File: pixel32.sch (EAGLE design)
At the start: 66 parts, among them CON1 DS1066-07M-SIDE, CON2 DS1066-07M-SIDE, CON3 PINHEAD_1X02-2.54, CON4 PINHEAD_1X01-2.54, CON5 PINHEAD_1X01-2.54, CON6 PINHEAD_1X01-2.54, CON7 PINHEAD_1X01-2.54, IC1 STM32F030K6TX-LQFP32(7X7), IC3 ST3485SOIC8, IC6 MC74VHC1GT125, IC7 MC74VHC1GT125, IC8 LM317

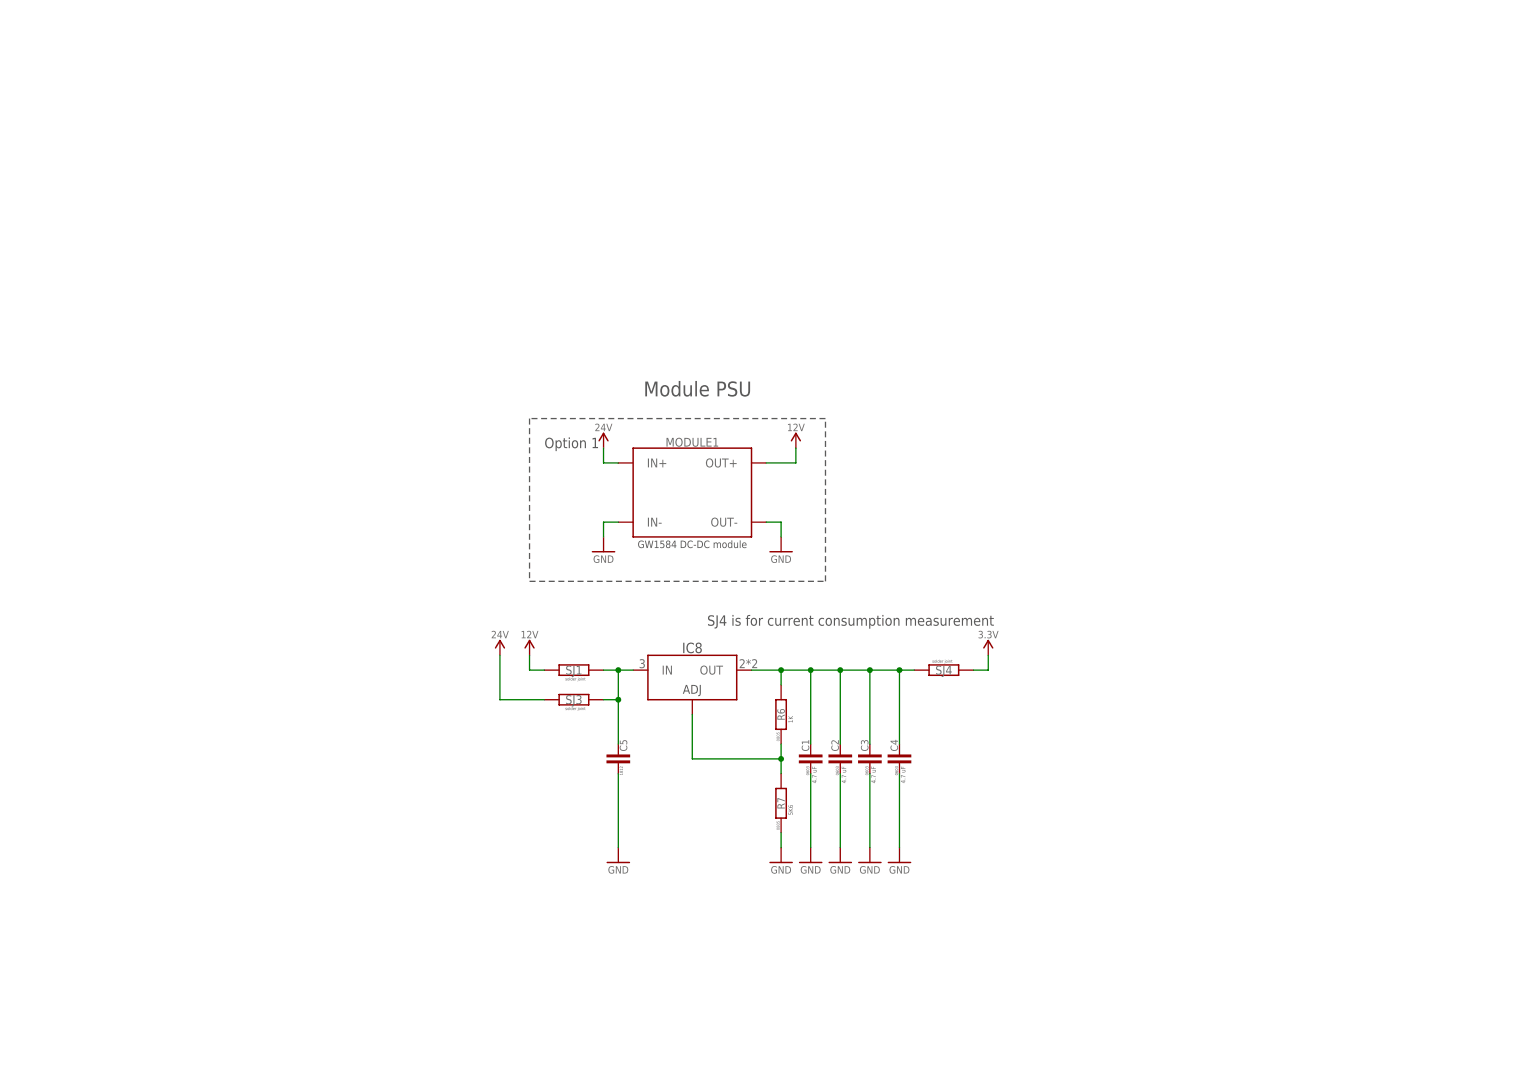
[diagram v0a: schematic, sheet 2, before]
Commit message: PCB Finalization #2
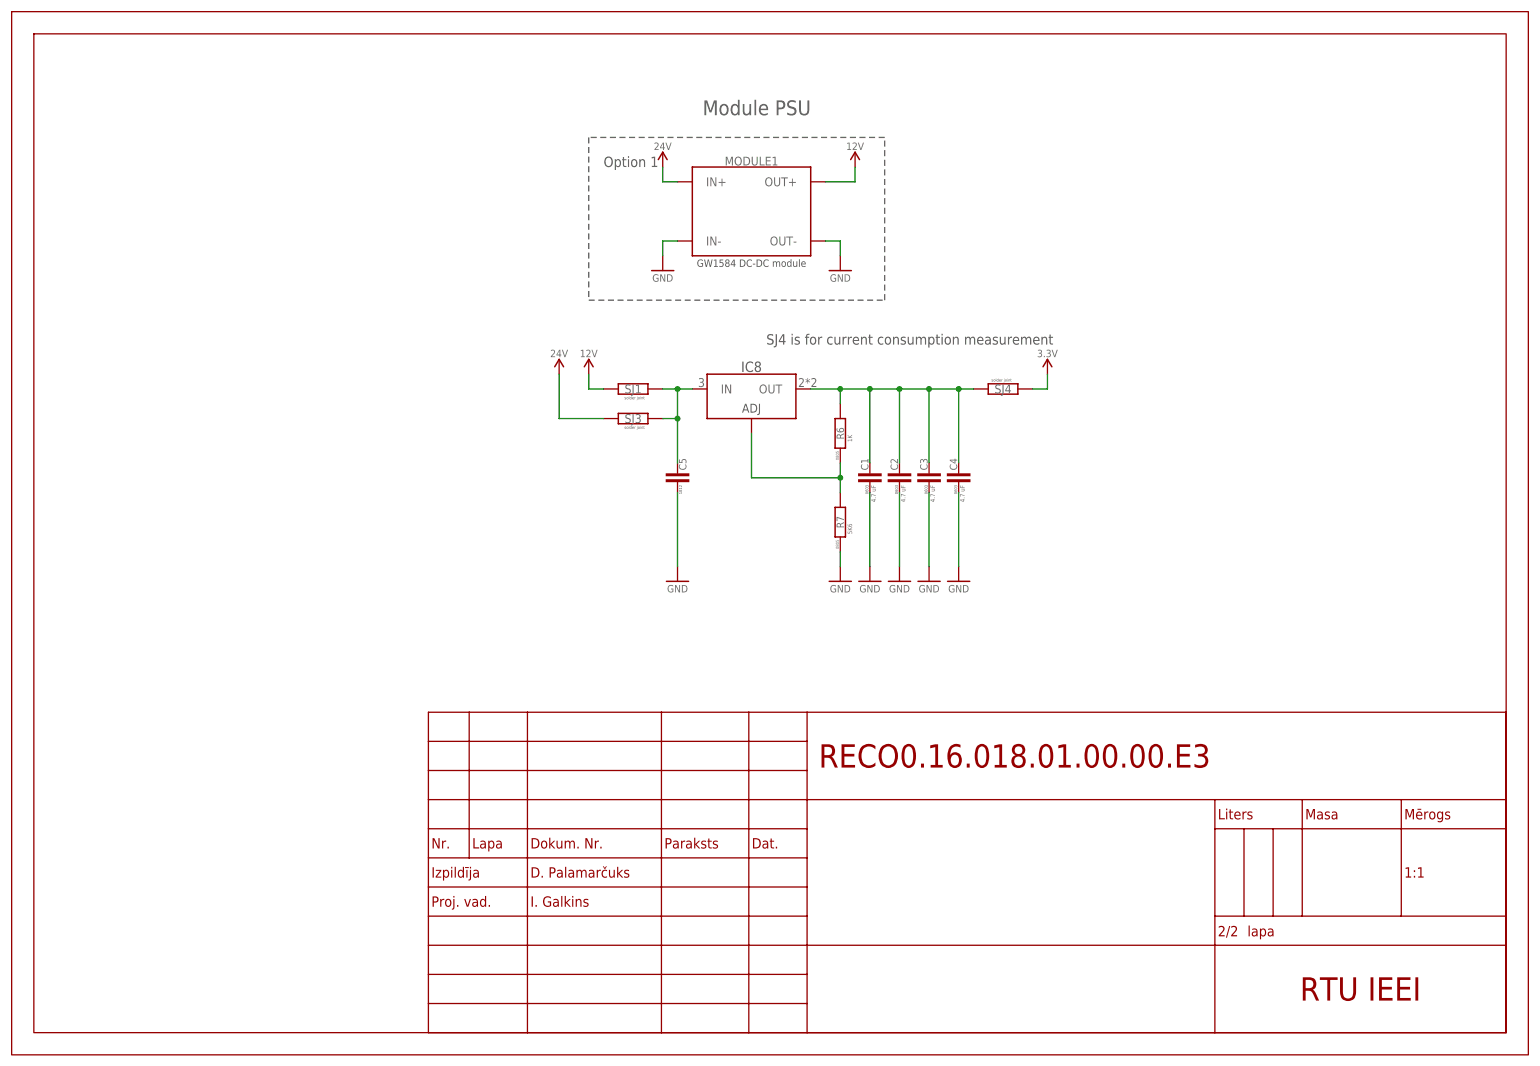
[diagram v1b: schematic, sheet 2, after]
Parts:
- added FRAME1: RTU_A4, frames:RTU_A4
- added FRAME2: RTU_A3, frames:RTU_A3
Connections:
- net LED1_CURRENT: now also IC1.PA6; no longer IC1.PA7/C1N
- net LED2_CURRENT: now also IC1.PA7/C1N; no longer IC1.PA6
- net LED3_CURRENT: now also IC1.PB0/C2N; no longer IC1.PA5
- net VIN_SENSE: now also IC1.PA5; no longer IC1.PB0/C2N
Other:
- moved on the sheet: C1, C2, C3, C4, C5, IC8, MODULE1, R6, R7, SJ1, SJ3, SJ4
